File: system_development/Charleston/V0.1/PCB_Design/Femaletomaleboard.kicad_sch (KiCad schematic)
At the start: 6 parts, among them J1 Screw_Terminal_01x12, J2 Screw_Terminal_01x12, J3 DB25_Receptacle

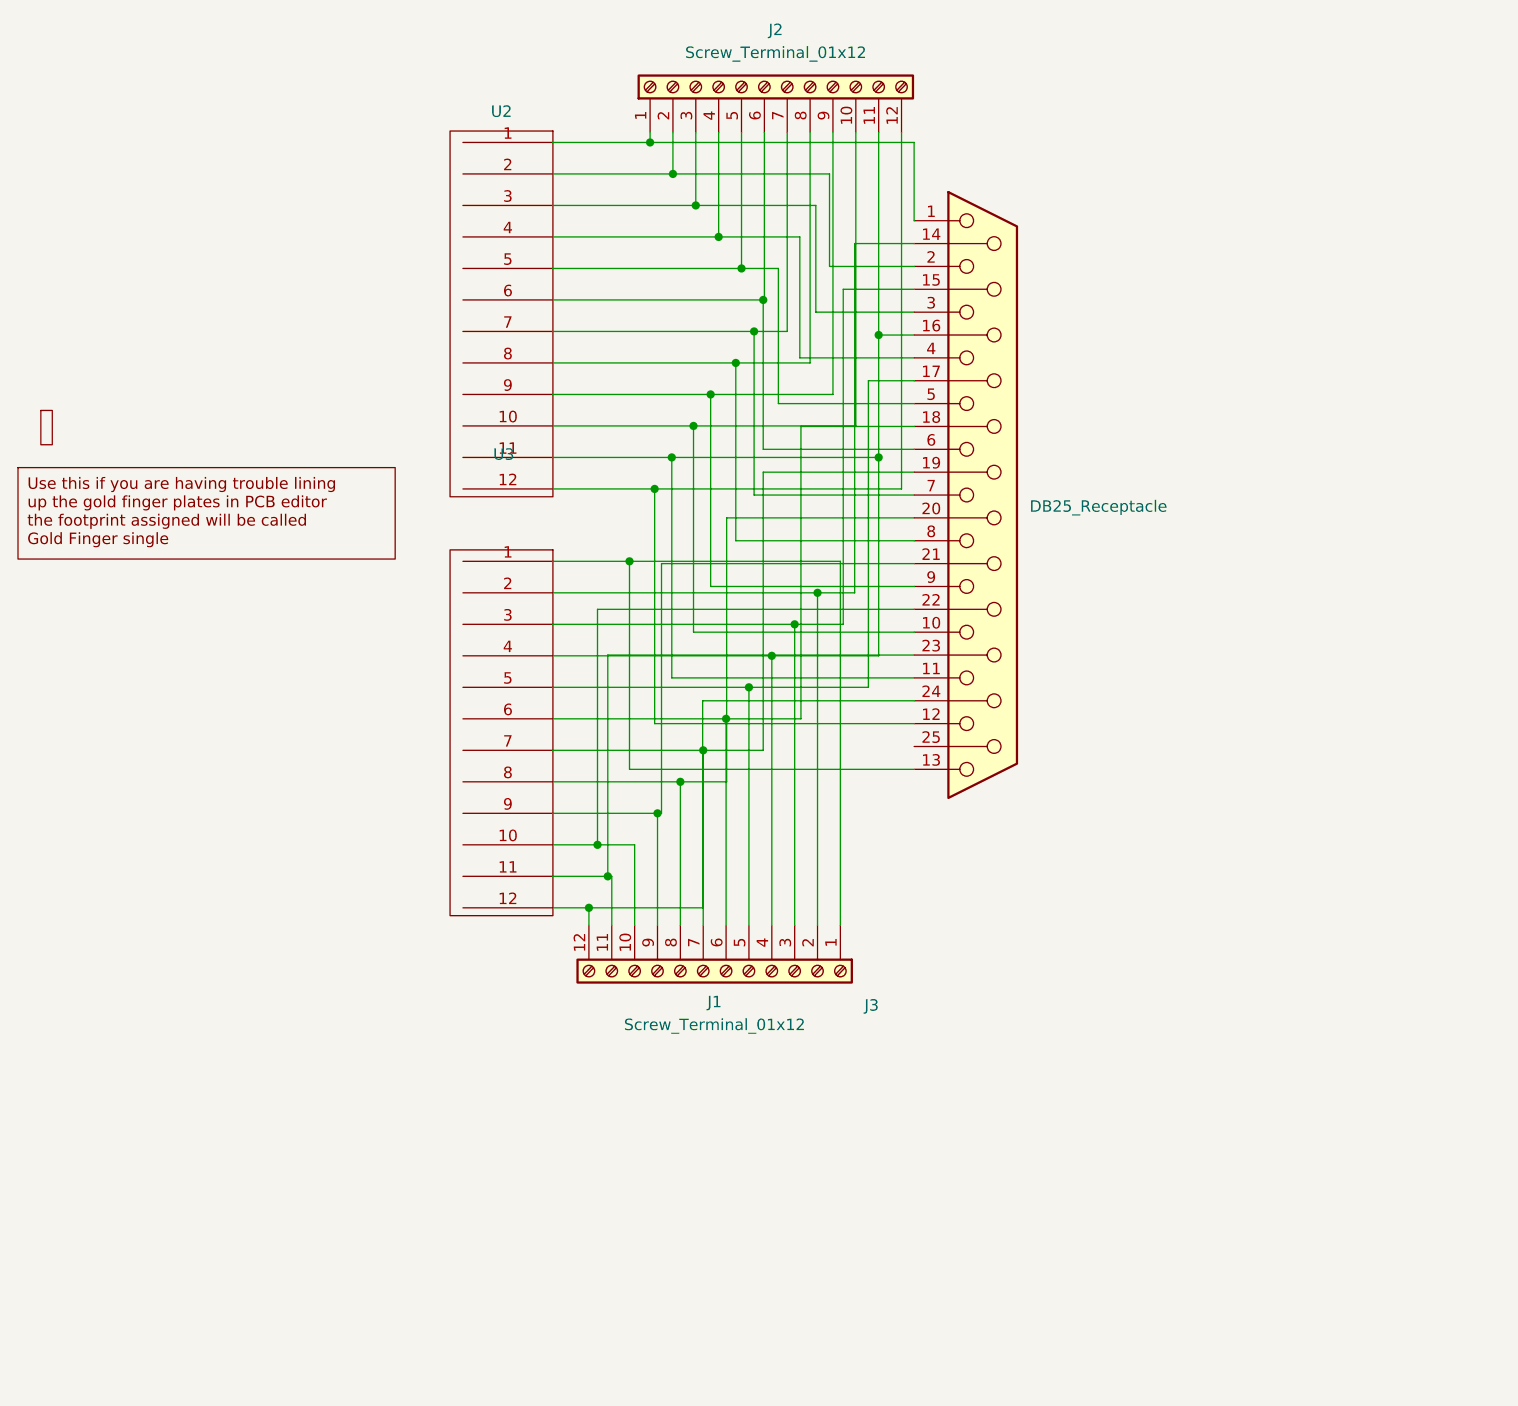
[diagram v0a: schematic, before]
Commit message: did it correctly with netlist and all.
Re did it with same desgin but with netlist and proper way
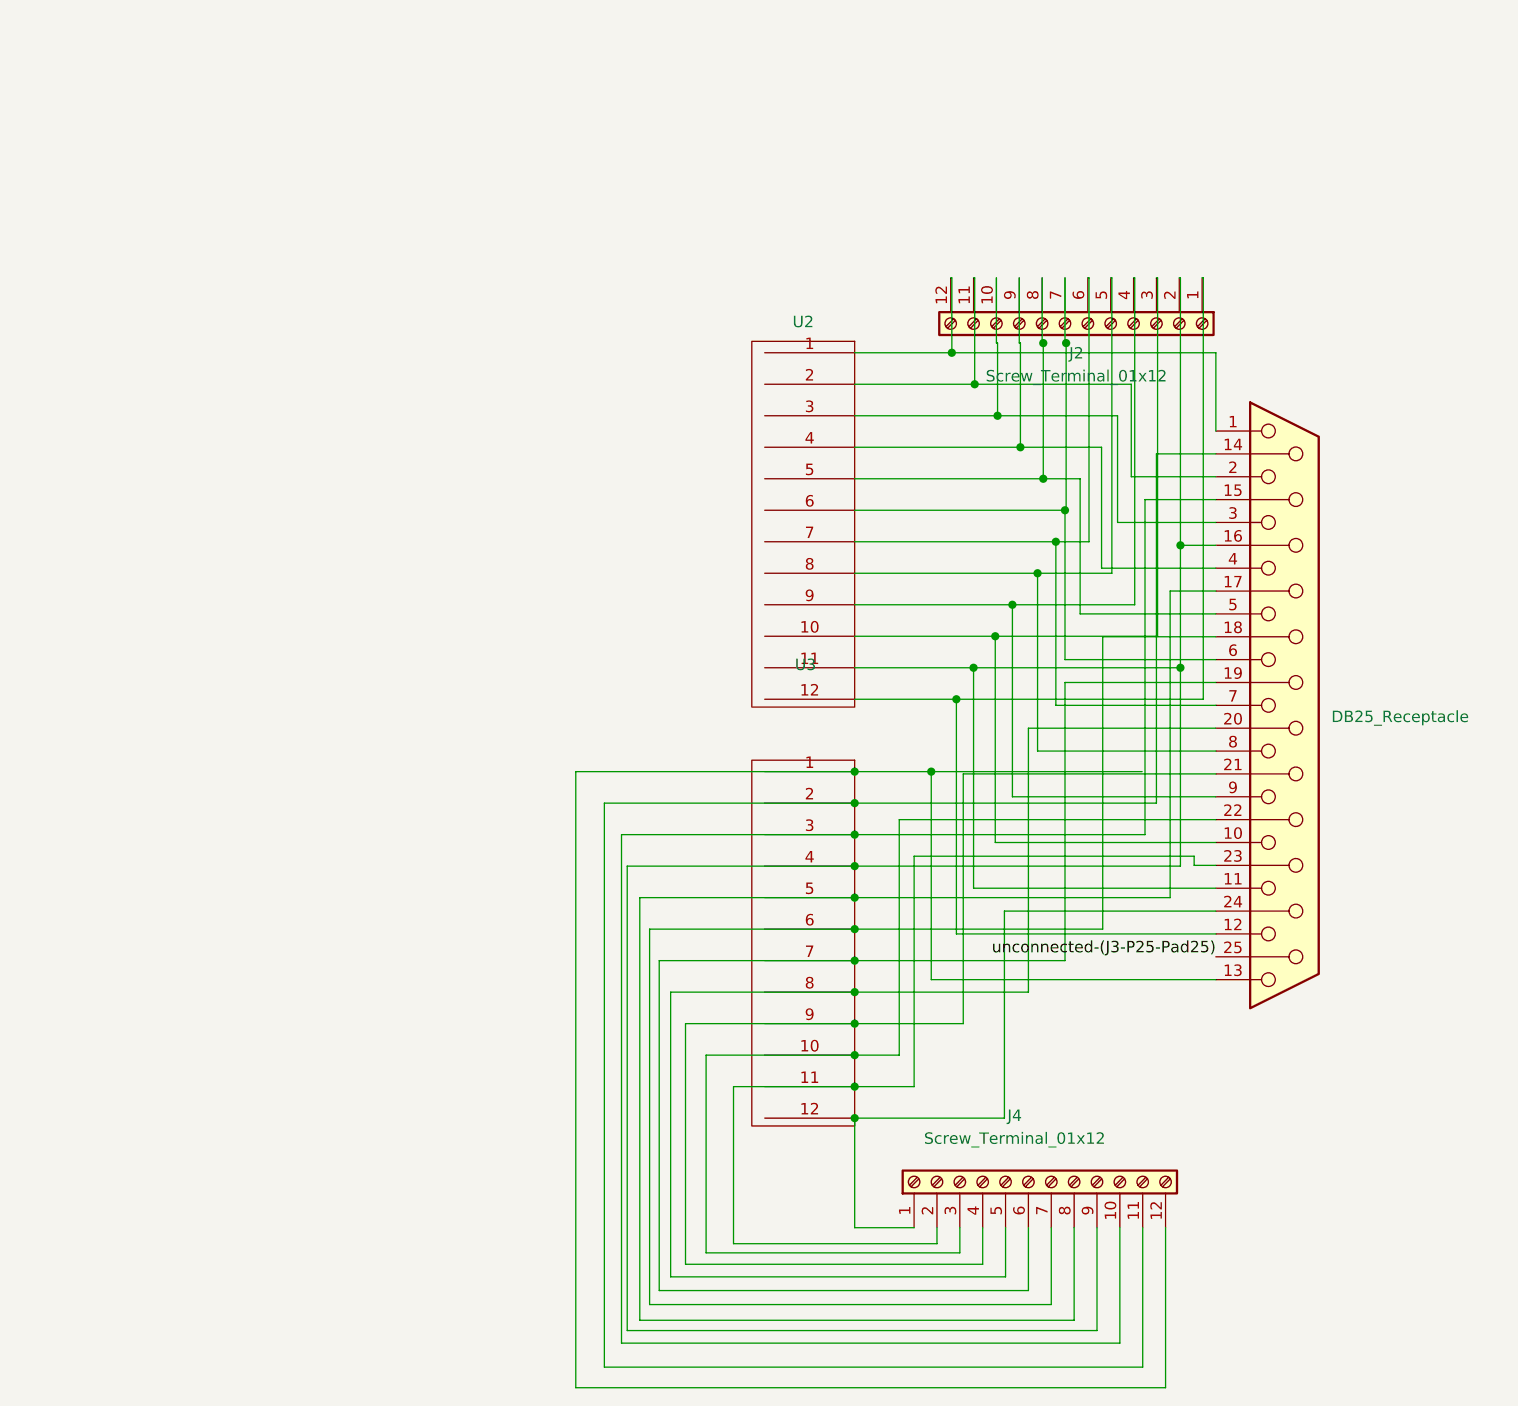
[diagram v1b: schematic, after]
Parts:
- removed J1: Screw_Terminal_01x12, infnoise_goldfingers:Gold Finger single, symbol libary_bms:Screw_Terminal_01x12
- removed U?: ~, symbol libary_bms:Goldfingersingle
- added J4: Screw_Terminal_01x12, TerminalBlock_Altech:Altech_AK300_1x12_P5.00mm_45-Degree, symbol screw_terminal_01x12:Screw_Terminal_01x12
- J3: footprint Connector_Dsub:DSUB-25_Male_Horizontal_P2.77x2.54mm_EdgePinOffset9.40mm -> Connector_Dsub:DSUB-25_Female_Horizontal_P2.77x2.54mm_EdgePinOffset9.40mm
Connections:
- net at J3.13, U3.1: now also J4.12 (Pin_12)
- net at J3.22 (P22), U3.10: now also J4.3 (Pin_3)
- net at J3.23 (P23), U3.11: now also J4.2 (Pin_2)
- net at J3.24 (P24), U3.12: now also J4.1 (Pin_1)
- net at J3.14 (P14), U3.2: now also J4.11 (Pin_11)
- net at J3.15 (P15), U3.3: now also J4.10 (Pin_10)
- net at J3.11, J3.16 (P16), U2.11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: now also J2.2 (Pin_2), J4.9 (Pin_9); no longer J2.11 (Pin_11)
- net at J3.17 (P17), U3.5: now also J4.8 (Pin_8)
- net at J3.18 (P18), U3.6: now also J4.7 (Pin_7)
- net at J3.19 (P19), U3.7: now also J4.6 (Pin_6)
- net at J3.20 (P20), U3.8: now also J4.5 (Pin_5)
- net at J3.21 (P21), U3.9: now also J4.4 (Pin_4)
- net at J3.1, U2.1: now also J2.12 (Pin_12); no longer J2.1 (Pin_1)
- net at J3.10, U2.10: now also J2.3 (Pin_3); no longer J2.10 (Pin_10)
- net at J3.12, U2.12: now also J2.1 (Pin_1); no longer J2.12 (Pin_12)
- net at J3.2, U2.2: now also J2.11 (Pin_11); no longer J2.2 (Pin_2)
- net unconnected-(J3-P25-Pad25): now reaches J3.25 (P25)
- net at J3.3, U2.3: now also J2.10 (Pin_10); no longer J2.3 (Pin_3)
- net at J3.4, U2.4: now also J2.9 (Pin_9); no longer J2.4 (Pin_4)
- net at J3.5, U2.5: now also J2.8 (Pin_8); no longer J2.5 (Pin_5)
- net at J3.6, U2.6: now also J2.7 (Pin_7); no longer J2.6 (Pin_6)
- net at J3.7, U2.7: now also J2.6 (Pin_6); no longer J2.7 (Pin_7)
- net at J3.8, U2.8: now also J2.5 (Pin_5); no longer J2.8 (Pin_8)
- net at J3.9, U2.9: now also J2.4 (Pin_4); no longer J2.9 (Pin_9)
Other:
- moved on the sheet: J2, U2, U3
